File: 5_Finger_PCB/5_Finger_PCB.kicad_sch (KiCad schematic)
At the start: 0 parts

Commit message: Update five finger PCB schematic
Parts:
- added C1: 10uF, symbol Device:C
- added C2, C4: 100nF, symbol Device:C
- added C3: 1uF, symbol Device:C
- added J1: Conn_01x06, symbol Connector_Generic:Conn_01x06
- added J2: USB_C_Receptacle_USB2.0_16P, symbol Connector:USB_C_Receptacle_USB2.0_16P
- added J3: DXL_MOTOR_1, Connector_JST:JST_EH_B3B-EH-A_1x03_P2.50mm_Vertical, symbol Connector_Generic:Conn_01x03
- added J4: DXL_MOTOR_2, Connector_JST:JST_EH_B3B-EH-A_1x03_P2.50mm_Vertical, symbol Connector_Generic:Conn_01x03
- added J5: DXL_MOTOR_3, Connector_JST:JST_EH_B3B-EH-A_1x03_P2.50mm_Vertical, symbol Connector_Generic:Conn_01x03
- added J6: DXL_MOTOR_4, Connector_JST:JST_EH_B3B-EH-A_1x03_P2.50mm_Vertical, symbol Connector_Generic:Conn_01x03
- added J7: DXL_MOTOR_5, Connector_JST:JST_EH_B3B-EH-A_1x03_P2.50mm_Vertical, symbol Connector_Generic:Conn_01x03
- added R1, R10, R2, R8, R9: 10k, symbol Device:R
- added R3, R4: 22, symbol Device:R
- added R5: 499, symbol Device:R
- added R6, R7: 5.1k, symbol Device:R
- added SW1: RESET, symbol Switch:SW_Push
- added SW2: BOOT, symbol Switch:SW_Push
- added U1: ESP32-S3-WROOM-1-N8R8, RF_Module:ESP32-S3-WROOM-1, symbol RF_Module:ESP32-S3-WROOM-1
- added U2: USBLC6-2SC6, Package_TO_SOT_SMD:SOT-23-6, symbol Power_Protection:USBLC6-2SC6
- added U3: 74LVC2G241, symbol 74xGxx:74LVC2G241
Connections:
- new net: J2.A5 (CC1), R6.1
- new net: J2.A6 (D+), J2.B6 (D+), U2.3 (I/O2)
- new net: J2.A7 (D-), J2.B7 (D-), U2.1 (I/O1)
- new net: J2.B5 (CC2), R7.1
- new net: R3.1, U1.13 (USB_D-)
- new net: R4.1, U1.14 (USB_D+)
- new net: R5.1, U1.37 (TXD0)
- new net DXL_DATA: J3.3 (Pin_3), J4.3 (Pin_3), J5.3 (Pin_3), J6.3 (Pin_3), J7.3 (Pin_3), R8.2, U3.2, U3.3
- new net DXL_TX_EN: R10.1, U1.23 (IO21), U3.1, U3.7
- new net DXL_UART_RX: R9.2, U1.11 (IO18), U3.6
- new net DXL_UART_TX: U1.10 (IO17), U3.5
- new net ESP_EN: C3.1, J1.5 (Pin_5), R1.2, U1.3 (EN)
- new net ESP_GPIO0: J1.6 (Pin_6), R2.2, SW2.2, U1.27 (IO0)
- new net GND: C1.2, C2.1, C3.2, C4.2, J1.2 (Pin_2), J2.A1 (GND), J2.A12 (GND), J2.B1 (GND), J2.B12 (GND), J2.SH (SHIELD), J3.1 (Pin_1), J4.1 (Pin_1), J5.1 (Pin_1), J6.1 (Pin_1), J7.1 (Pin_1), R10.2, R6.2, R7.2, SW1.1, SW1.2, SW2.1, U1.1 (GND), U1.40 (GND), U1.41 (GND), U2.2 (GND), U3.4 (GND)
- new net LOGIC_3V3: C1.1, C2.2, C4.1, J1.1 (Pin_1), R1.1, R2.1, R8.1, R9.1, U1.2 (3V3), U3.8 (VCC)
- new net MOTOR_5V: J3.2 (Pin_2), J4.2 (Pin_2), J5.2 (Pin_2), J6.2 (Pin_2), J7.2 (Pin_2)
- new net UART0_RX: J1.4 (Pin_4), U1.36 (RXD0)
- new net UART0_TX: J1.3 (Pin_3), R5.2
- new net USB_D+: R4.2, U2.4 (I/O2)
- new net USB_D-: R3.2, U2.6 (I/O1)
- new net USB_VBUS: J2.A4 (VBUS), J2.A9 (VBUS), J2.B4 (VBUS), J2.B9 (VBUS), U2.5 (VBUS)
- no-connect marks 0 -> 5

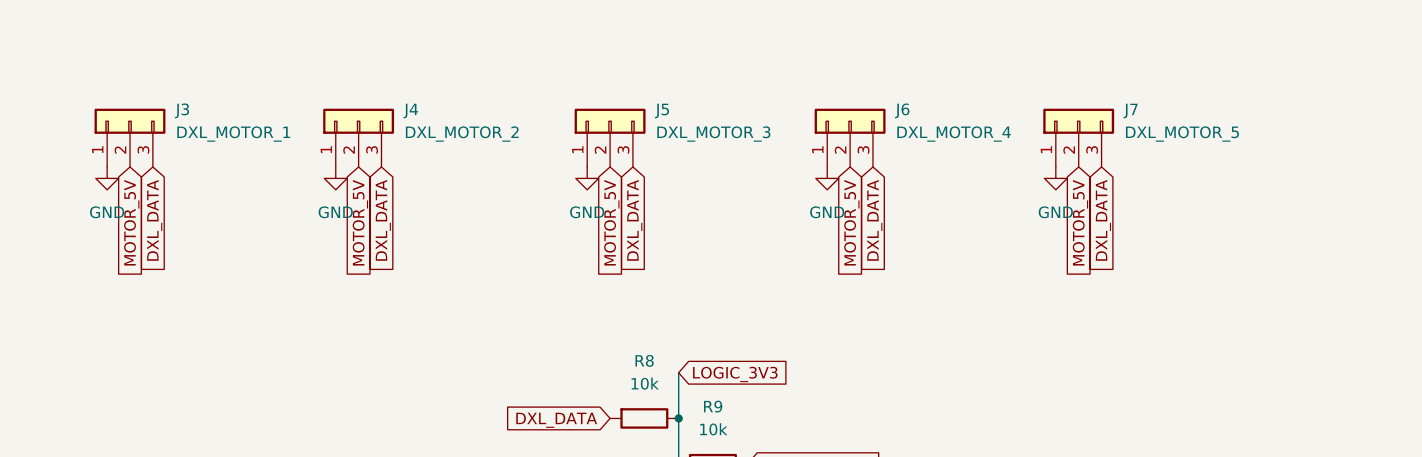
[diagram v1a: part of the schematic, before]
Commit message: Update KiCad schematic
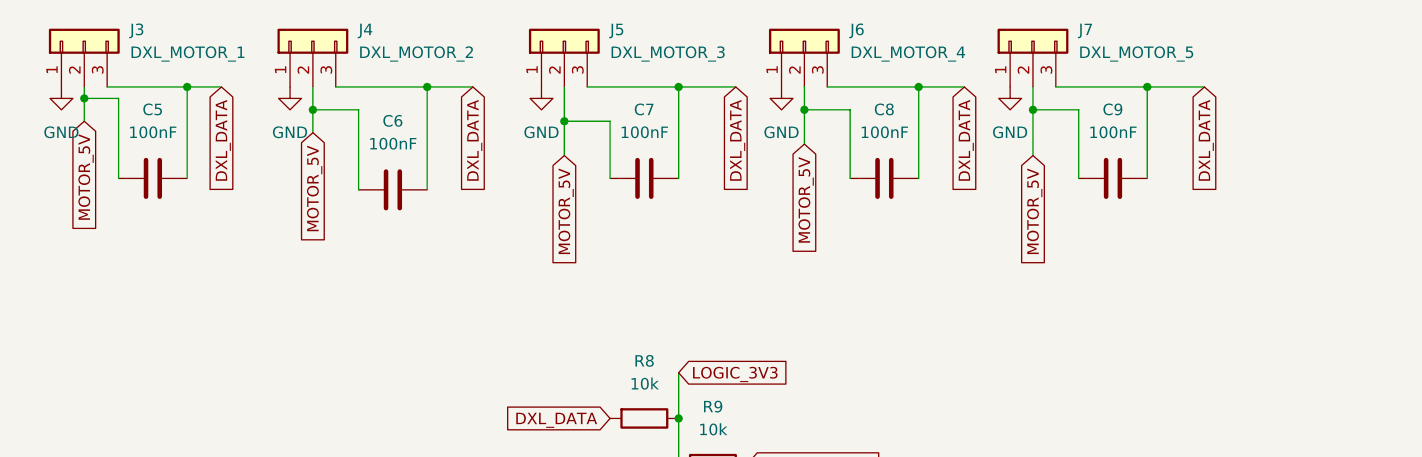
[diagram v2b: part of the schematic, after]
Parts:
- added C5, C6, C7, C8, C9: 100nF, symbol Device:C
- added unit 1 of U3
- added unit 2 of U3
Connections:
- net DXL_DATA: now also C5.2, C6.2, C7.2, C8.2, C9.2, U3.2, U3.3; no longer U3.2, U3.3
- net DXL_TX_EN: now also U3.1, U3.7; no longer U3.1, U3.7
- net DXL_UART_RX: now also U3.6; no longer U3.6
- net DXL_UART_TX: now also U3.5; no longer U3.5
- net MOTOR_5V: now also C5.1, C6.1, C7.1, C8.1, C9.1
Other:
- moved on the sheet: J3, J4, J5, J6, J7
